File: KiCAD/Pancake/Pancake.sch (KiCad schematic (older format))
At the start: 50 parts, among them IC3 LF347N, J1 Conn_01x08_Male, J101 TB001-500-04BE, J102 TB001-500-03BE, J2 Conn_01x08_Male, J3 Conn_01x08_Male, J4 Conn_01x08_Male, J5 Conn_01x08_Male, J7 Conn_02x15_Top_Bottom

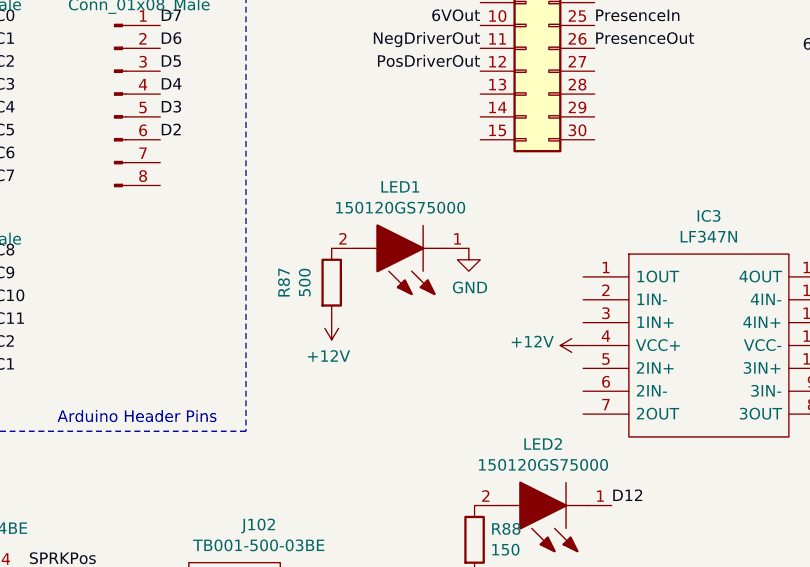
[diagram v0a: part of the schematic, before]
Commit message: Revising one last time before ordering
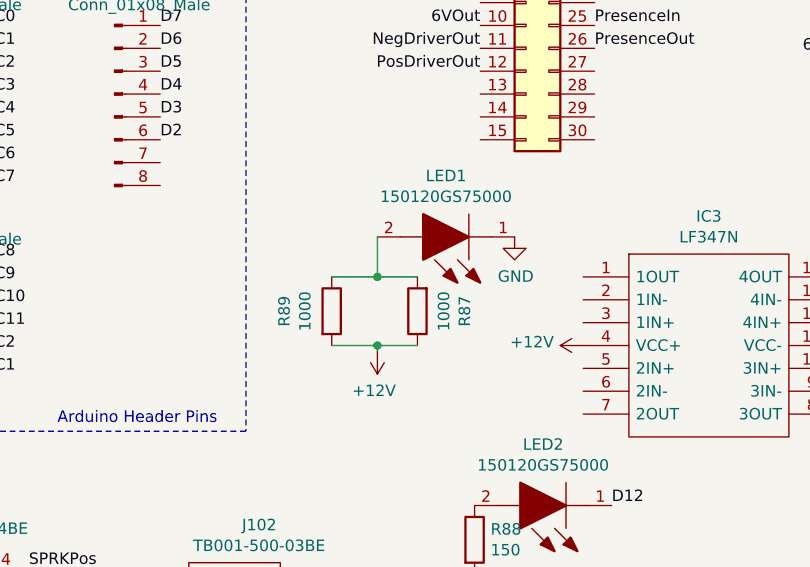
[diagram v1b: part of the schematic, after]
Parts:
- added R89: 1000, Resistor_SMD:R_1206_3216Metric_Pad1.30x1.75mm_HandSolder, symbol Device:R
- R87: value 500 -> 1000
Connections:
- net +12V: now also R87.1, R89.2; no longer R87.2
- net at LED1.2: now also R87.2, R89.1; no longer R87.1
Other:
- moved on the sheet: LED1, R87
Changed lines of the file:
@@
 L SamacSys_Parts:150120GS75000 LED1
 U 1 1 61471F94
-P 3225 2850
-F 0 "LED1" H 3525 2583 50  0000 C CNN
-F 1 "150120GS75000" H 3525 2674 50  0000 C CNN
-F 2 "SamacSys_Parts:LEDC3214X78N" H 3725 3000 50  0001 L BNN
-F 3 "https://docs-emea.rs-online.com/webdocs/1302/0900766b81302e28.pdf" H 3725 2900 50  0001 L BNN
-F 4 "LED,Wurth Elektronik,150120GS75000 Wurth Elektronik 150120GS75000, WL-SMCW Series Green LED, 520 nm, 3016 (1206) Clear, Rectangle Lens SMD Package" H 3725 2800 50  0001 L BNN "Description"
-F 5 "0.78" H 3725 2700 50  0001 L BNN "Height"
-F 6 "Wurth Elektronik" H 3725 2600 50  0001 L BNN "Manufacturer_Name"
-F 7 "150120GS75000" H 3725 2500 50  0001 L BNN "Manufacturer_Part_Number"
-F 8 "710-150120GS75000" H 3725 2400 50  0001 L BNN "Mouser Part Number"
-F 9 "https://www.mouser.co.uk/ProductDetail/Wurth-Elektronik/150120GS75000?qs=LlUlMxKIyB3I3AMxrmBw4A%3D%3D" H 3725 2300 50  0001 L BNN "Mouser Price/Stock"
-F 10 "" H 3725 2200 50  0001 L BNN "Arrow Part Number"
-F 11 "" H 3725 2100 50  0001 L BNN "Arrow Price/Stock"
-	1    3225 2850
+P 3425 2800
+F 0 "LED1" H 3725 2533 50  0000 C CNN
+F 1 "150120GS75000" H 3725 2624 50  0000 C CNN
+F 2 "SamacSys_Parts:LEDC3214X78N" H 3925 2950 50  0001 L BNN
+F 3 "https://docs-emea.rs-online.com/webdocs/1302/0900766b81302e28.pdf" H 3925 2850 50  0001 L BNN
+F 4 "LED,Wurth Elektronik,150120GS75000 Wurth Elektronik 150120GS75000, WL-SMCW Series Green LED, 520 nm, 3016 (1206) Clear, Rectangle Lens SMD Package" H 3925 2750 50  0001 L BNN "Description"
+F 5 "0.78" H 3925 2650 50  0001 L BNN "Height"
+F 6 "Wurth Elektronik" H 3925 2550 50  0001 L BNN "Manufacturer_Name"
+F 7 "150120GS75000" H 3925 2450 50  0001 L BNN "Manufacturer_Part_Number"
+F 8 "710-150120GS75000" H 3925 2350 50  0001 L BNN "Mouser Part Number"
+F 9 "https://www.mouser.co.uk/ProductDetail/Wurth-Elektronik/150120GS75000?qs=LlUlMxKIyB3I3AMxrmBw4A%3D%3D" H 3925 2250 50  0001 L BNN "Mouser Price/Stock"
+F 10 "" H 3925 2150 50  0001 L BNN "Arrow Part Number"
+F 11 "" H 3925 2050 50  0001 L BNN "Arrow Price/Stock"
+	1    3425 2800
 	-1   0    0    1
 $EndComp
@@
 L Device:R R?
 U 1 1 6147D62C
-P 2625 3000
+P 3000 3125
 AR Path="/61024B6A/6147D62C" Ref="R?"  Part="1"
 AR Path="/612AE90B/6147D62C" Ref="R?"  Part="1"
 AR Path="/6147D62C" Ref="R87"  Part="1"
-F 0 "R87" V 2418 3000 50  0000 C CNN
-F 1 "500" V 2509 3000 50  0000 C CNN
-F 2 "Resistor_SMD:R_1206_3216Metric_Pad1.30x1.75mm_HandSolder" V 2555 3000 50  0001 C CNN
-F 3 "~" H 2625 3000 50  0001 C CNN
-	1    2625 3000
-	1    0    0    -1
+F 0 "R87" V 2793 3125 50  0000 C CNN
+F 1 "1000" V 2884 3125 50  0000 C CNN
+F 2 "Resistor_SMD:R_1206_3216Metric_Pad1.30x1.75mm_HandSolder" V 2930 3125 50  0001 C CNN
+F 3 "~" H 3000 3125 50  0001 C CNN
+	1    3000 3125
+	-1   0    0    1
 $EndComp
 $Comp
 L power:+12V #PWR01
 U 1 1 61484A8A
-P 2625 3150
-F 0 "#PWR01" H 2625 3000 50  0001 C CNN
-F 1 "+12V" H 2640 3323 50  0000 C CNN
-F 2 "" H 2625 3150 50  0001 C CNN
-F 3 "" H 2625 3150 50  0001 C CNN
-	1    2625 3150
+P 2825 3300
+F 0 "#PWR01" H 2825 3150 50  0001 C CNN
+F 1 "+12V" H 2840 3473 50  0000 C CNN
+F 2 "" H 2825 3300 50  0001 C CNN
+F 3 "" H 2825 3300 50  0001 C CNN
+	1    2825 3300
 	-1   0    0    1
 $EndComp
@@
 L power:GND #PWR02
 U 1 1 61485A09
-P 3225 2850
-F 0 "#PWR02" H 3225 2600 50  0001 C CNN
-F 1 "GND" H 3230 2677 50  0000 C CNN
-F 2 "" H 3225 2850 50  0001 C CNN
-F 3 "" H 3225 2850 50  0001 C CNN
-	1    3225 2850
+P 3425 2800
+F 0 "#PWR02" H 3425 2550 50  0001 C CNN
+F 1 "GND" H 3430 2627 50  0000 C CNN
+F 2 "" H 3425 2800 50  0001 C CNN
+F 3 "" H 3425 2800 50  0001 C CNN
+	1    3425 2800
 	1    0    0    -1
 $EndComp
@@
 	1    0    0    -1
 $EndComp
+$Comp
+L Device:R R?
+U 1 1 614E4DCA
+P 2625 3125
+AR Path="/61024B6A/614E4DCA" Ref="R?"  Part="1"
+AR Path="/612AE90B/614E4DCA" Ref="R?"  Part="1"
+AR Path="/614E4DCA" Ref="R89"  Part="1"
+F 0 "R89" V 2418 3125 50  0000 C CNN
+F 1 "1000" V 2509 3125 50  0000 C CNN
+F 2 "Resistor_SMD:R_1206_3216Metric_Pad1.30x1.75mm_HandSolder" V 2555 3125 50  0001 C CNN
+F 3 "~" H 2625 3125 50  0001 C CNN
+	1    2625 3125
+	1    0    0    -1
+$EndComp
+Wire Wire Line
+	2825 3300 2825 3275
+Wire Wire Line
+	2825 3275 3000 3275
+Wire Wire Line
+	2625 3275 2825 3275
+Connection ~ 2825 3275
+Wire Wire Line
+	2625 2975 2825 2975
+Wire Wire Line
+	2825 2800 2825 2975
+Connection ~ 2825 2975
+Wire Wire Line
+	2825 2975 3000 2975
 $EndSCHEMATC
